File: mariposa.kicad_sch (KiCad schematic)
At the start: 27 parts, among them J1 Conn_01x22_Shielded, J2 Conn_01x03_MountingPin, J3 Conn_ARM_SWD_TagConnect_TC203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, J5 Conn_02x03_Counter_Clockwise, J6 Conn_01x05_Socket, SW1 SW_Push, SW3 SW_Push

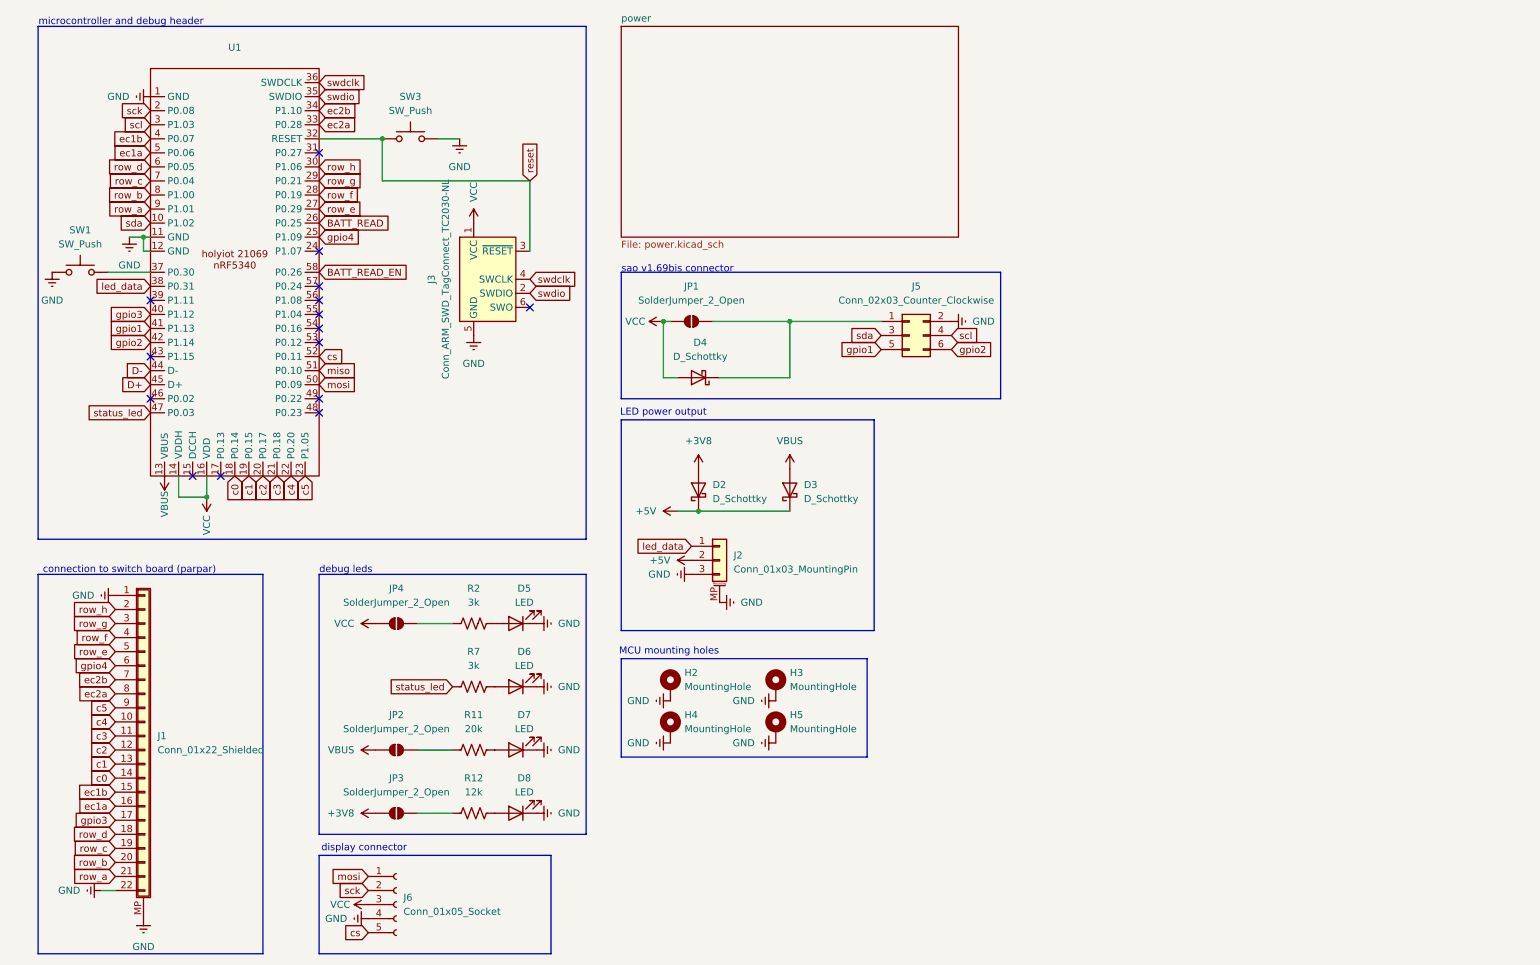
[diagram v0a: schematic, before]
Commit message: mariposa v2 RC2
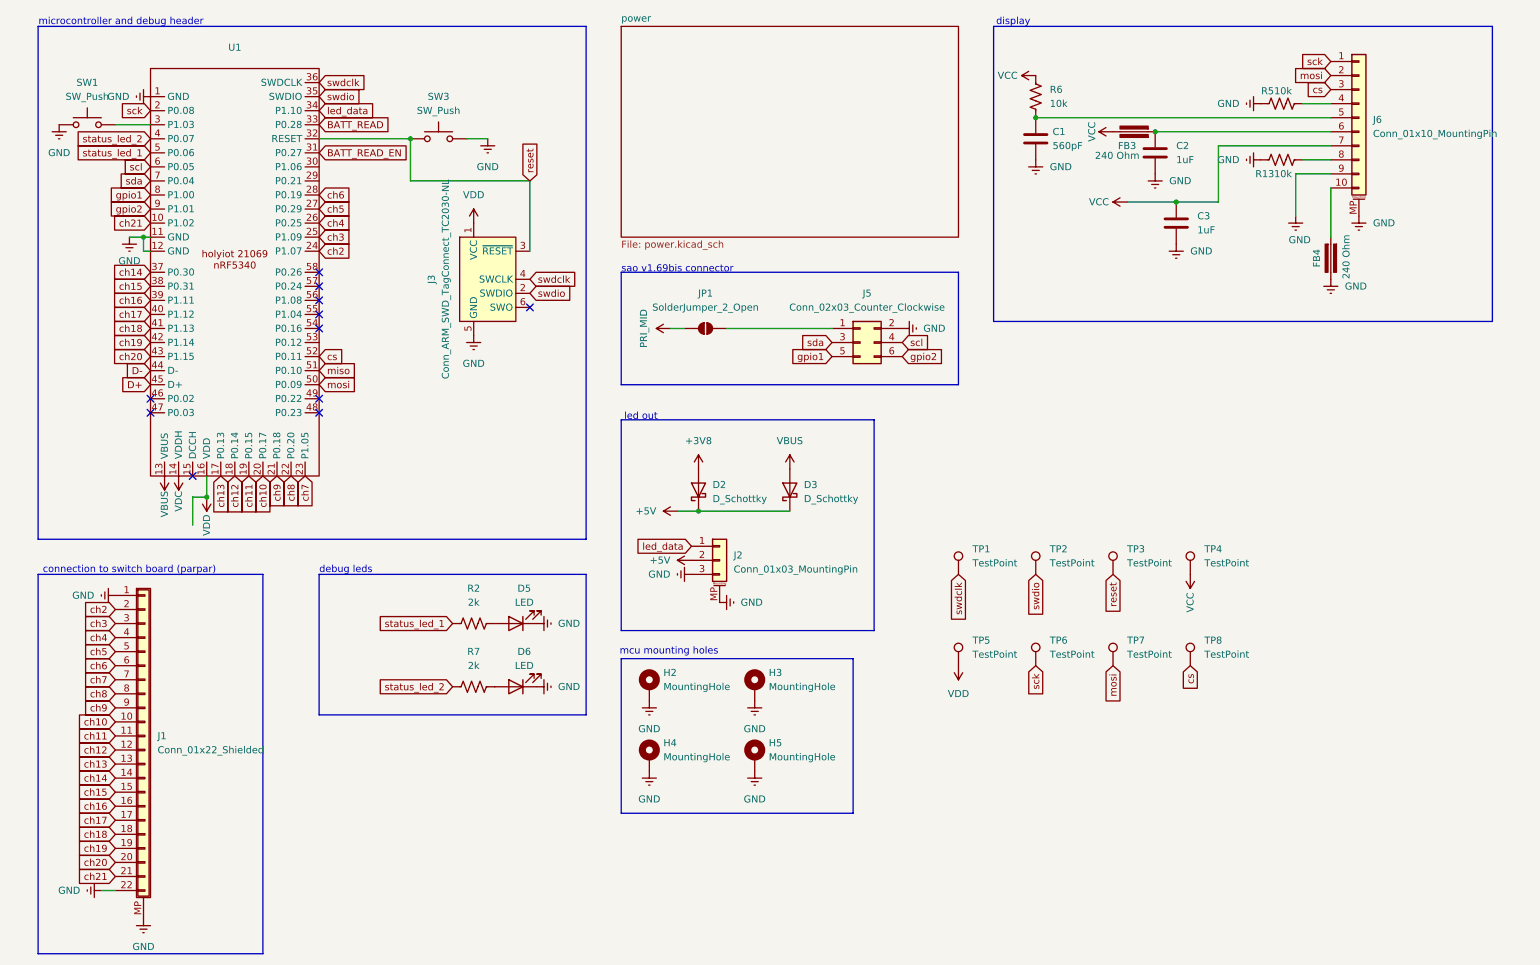
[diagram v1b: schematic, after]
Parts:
- removed D4: D_Schottky, PCM_Diode_SMD_Handsoldering_AKL:D_SOD-123F, symbol Device:D_Schottky
- removed D7, D8: LED, LED_SMD:LED_0805_2012Metric, symbol Device:LED
- removed J6: Conn_01x05_Socket, coquette_footprints:5-pin horizontal display, symbol Connector:Conn_01x05_Socket
- removed JP2, JP3, JP4: SolderJumper_2_Open, Jumper:SolderJumper-2_P1.3mm_Open_TrianglePad1.0x1.5mm, symbol Jumper:SolderJumper_2_Open
- removed R11: 20k, Resistor_SMD:R_0603_1608Metric, symbol Device:R_US
- removed R12: 12k, Resistor_SMD:R_0603_1608Metric, symbol Device:R_US
- added C1: 560pF, Capacitor_SMD:C_0603_1608Metric, symbol Device:C
- added C2, C3: 1uF, Capacitor_SMD:C_0603_1608Metric, symbol Device:C
- added FB3, FB4: 240 Ohm, PCM_Ferrite_SMD_AKL:Ferrite_0603_1608Metric, symbol PCM_Device_AKL:Ferrite_Bead
- added J6: Conn_01x10_MountingPin, Connector_FFC-FPC:Hirose_FH12-10S-0.5SH_1x10-1MP_P0.50mm_Horizontal, symbol Connector_Generic_MountingPin:Conn_01x10_MountingPin
- added R13, R5, R6: 10k, Resistor_SMD:R_0603_1608Metric, symbol Device:R_US
- added TP1, TP2, TP3, TP4, TP5, TP6, TP7, TP8: TestPoint, TestPoint:TestPoint_Pad_D1.0mm, symbol Connector:TestPoint
- D5, D6: footprint LED_SMD:LED_0805_2012Metric -> LED_SMD:LED_1206_3216Metric_ReverseMount_Hole1.8x2.4mm
- J2: footprint Connector_JST:JST_PH_S3B-PH-SM4-TB_1x03-1MP_P2.00mm_Horizontal -> Connector_JST:JST_SH_SM03B-SRSS-TB_1x03-1MP_P1.00mm_Horizontal
- R2, R7: value 3k -> 2k
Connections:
- net BATT_READ: now also U1.33 (P0.28); no longer U1.26 (P0.25)
- net BATT_READ_EN: now also U1.31 (P0.27); no longer U1.58 (P0.26)
- net GND: now also C1.2, C2.2, C3.2, FB4.2, J6.9 (Pin_9), J6.MP (MountPin), R13.1, R5.1
- net VCC: now also C3.1, FB3.2, J6.7 (Pin_7), R6.2, TP4.1; no longer J3.1 (VCC), JP1.1 (A), U1.14 (VDDH), U1.16 (VDD)
- net cs: now also J6.3 (Pin_3), TP8.1
- net gpio1: now also U1.8 (P1.00); no longer U1.41 (P1.13)
- net gpio2: now also U1.9 (P1.01); no longer U1.42 (P1.14)
- net led_data: now also U1.34 (P1.10); no longer U1.38 (P0.31)
- net mosi: now also J6.2 (Pin_2), TP7.1
- net reset: now also TP3.1
- net sck: now also J6.1 (Pin_1), TP6.1
- net scl: now also U1.6 (P0.05); no longer U1.3 (P1.03)
- net sda: now also U1.7 (P0.04); no longer U1.10 (P1.02)
- net swdclk: now also TP1.1
- net swdio: now also TP2.1
- net status_led_1: now reaches R2.2
- net status_led_1: now also U1.5 (P0.06)
- net ch13: now reaches U1.17 (P0.13)
- net ch13: now also J1.13 (Pin_13)
- net ch2: now reaches U1.24 (P1.07)
- net ch2: now also J1.2 (Pin_2)
- net at SW1.2: now also U1.3 (P1.03); no longer U1.37 (P0.30)
- net ch16: now reaches U1.39 (P1.11)
- net ch16: now also J1.16 (Pin_16)
- net ch20: now reaches U1.43 (P1.15)
- net ch20: now also J1.20 (Pin_20)
- net c0 renamed ch12
- net ch12: now also J1.12 (Pin_12); no longer J1.14 (Pin_14)
- net c1 renamed ch11
- net ch11: now also J1.11 (Pin_11); no longer J1.13 (Pin_13)
- net c2 renamed ch10
- net ch10: now also J1.10 (Pin_10); no longer J1.12 (Pin_12)
- net c3 renamed ch9
- net ch9: now also J1.9 (Pin_9); no longer J1.11 (Pin_11)
- net c4 renamed ch8
- net ch8: now also J1.8 (Pin_8); no longer J1.10 (Pin_10)
- net c5 renamed ch7
- net ch7: now also J1.7 (Pin_7); no longer J1.9 (Pin_9)
- removed net ec1a: J1.16 (Pin_16), U1.5 (P0.06)
- net ec1b renamed ch15
- net ch15: now also U1.38 (P0.31); no longer U1.4 (P0.07)
- removed net ec2a: J1.8 (Pin_8), U1.33 (P0.28)
- removed net ec2b: J1.7 (Pin_7), U1.34 (P1.10)
- net gpio3 renamed ch17
- net gpio4 renamed ch3
- net ch3: now also J1.3 (Pin_3); no longer J1.6 (Pin_6)
- net row_a renamed ch21
- net ch21: now also U1.10 (P1.02); no longer U1.9 (P1.01)
- removed net row_b: J1.20 (Pin_20), U1.8 (P1.00)
- net row_c renamed ch19
- net ch19: now also U1.42 (P1.14); no longer U1.7 (P0.04)
- net row_d renamed ch18
- net ch18: now also U1.41 (P1.13); no longer U1.6 (P0.05)
- net row_e renamed ch5
- net row_f renamed ch4
- net ch4: now also U1.26 (P0.25); no longer U1.28 (P0.19)
- net row_g: no longer names the net of U1.29 (P0.21)
- net row_g: no longer J1.3 (Pin_3)
- net row_h: no longer names the net of U1.30 (P1.06)
- net row_h: no longer J1.2 (Pin_2)
- net status_led: no longer names the net of U1.47 (P0.03)
- net status_led: no longer R7.2
- new net: C1.1, J6.5 (Pin_5), R6.1
- new net: J6.4 (Pin_4), R5.2
- new net: FB4.1, J6.10 (Pin_10)
- new net: C2.1, FB3.1, J6.6 (Pin_6)
- new net: J6.8 (Pin_8), R13.2
- new net PRI_MID: JP1.1 (A)
- new net VDC: U1.14 (VDDH)
- new net VDD: J3.1 (VCC), TP5.1, U1.16 (VDD)
- new net ch14: J1.14 (Pin_14), U1.37 (P0.30)
- new net ch6: J1.6 (Pin_6), U1.28 (P0.19)
- new net status_led_2: R7.2, U1.4 (P0.07)
- no-connect marks 15 -> 11
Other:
- note added: "display"
- note added: "led out"
- note added: "mcu mounting holes"
- note removed: "LED power output"
- note removed: "MCU mounting holes"
- note removed: "display connector"
- moved on the sheet: H2, H3, H4, H5, J5, JP1, SW1, SW3
